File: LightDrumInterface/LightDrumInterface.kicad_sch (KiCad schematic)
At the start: 63 parts, among them J1 MIDI-IN, J2 DEBUG-CONN, J3 MIDI-OUT, J4 PWR-CONN, J5 0525593652, J6 0541323662, Q101 NX6008NBKWX, Q102 NX6008NBKWX, Q103 NX6008NBKWX, Q104 NX6008NBKWX, SW1 RESET-SW, U1 STP16CP05, U2 TPL0401B-10-Q1, U3 74AUP2G04, U4 PC817

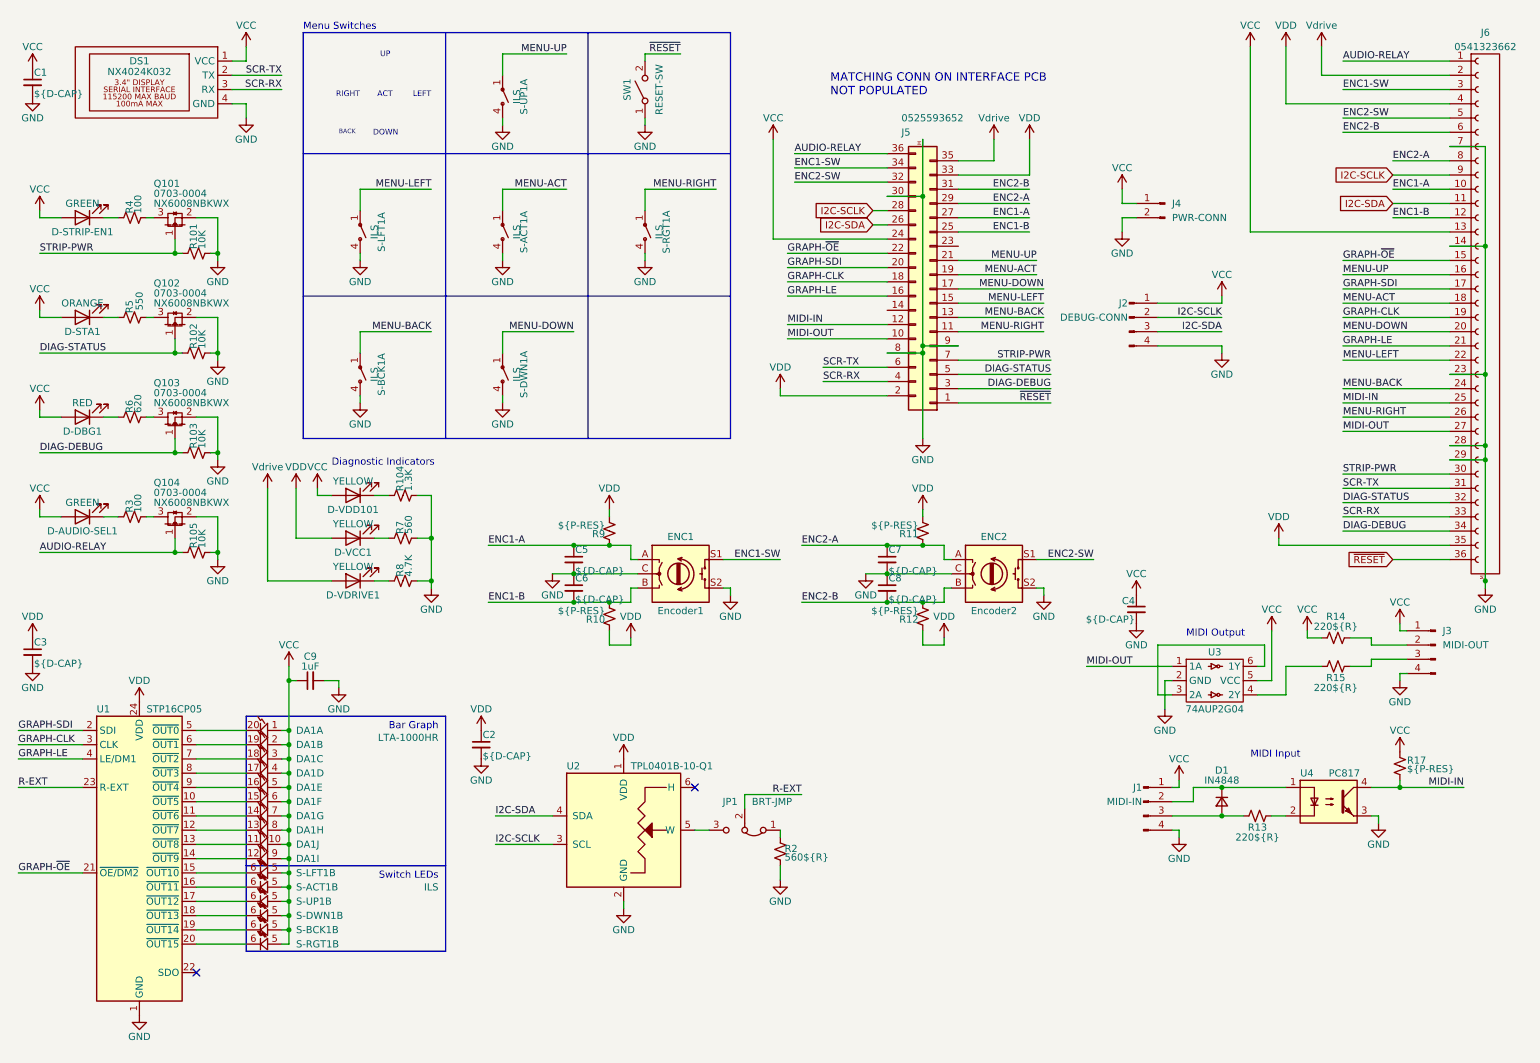
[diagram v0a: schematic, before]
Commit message: interface layout completed - REV6
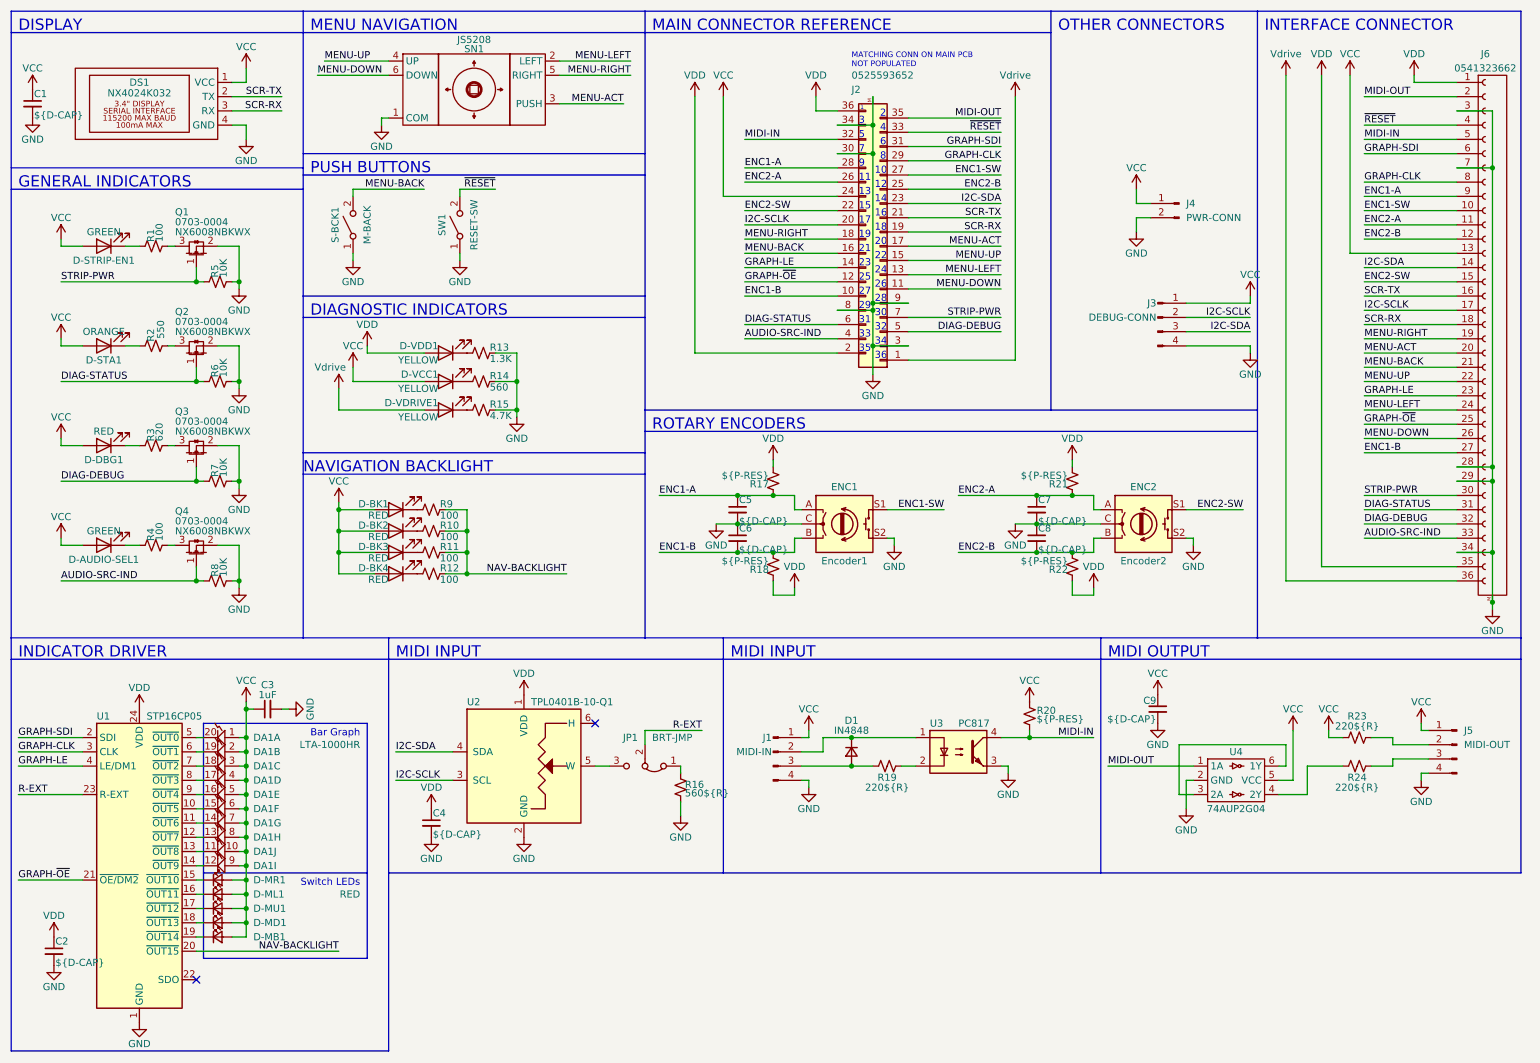
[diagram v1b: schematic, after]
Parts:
- removed S-ACT1, S-BCK1, S-DWN1, S-LFT1, S-RGT1, S-UP1: ILS, Daxxn_Switches:ILS-TB, symbol Daxxn_Buttons:ILS
- added D-BK1, D-BK2, D-BK3, D-BK4: RED, LED_SMD:LED_0805_2012Metric, symbol Device:LED
- added D-MB1, D-MD1, D-ML1, D-MR1, D-MU1: RED, LED_SMD:LED_0805_2012Metric, symbol Device:LED_Small
- added R10, R11, R12, R9: 100, Resistor_SMD:R_0805_2012Metric, symbol Device:R_Small_US
- added S-BCK1: M-BACK, Daxxn_Switches:TL3365AF180QG, symbol Switch:SW_SPST
- added SN1: JS5208, Daxxn_Switches:JS5208, symbol Daxxn_Buttons:JS5208
- DS1: footprint Daxxn_Displays:NX4024T032_10mm -> Daxxn_Displays:NX4024K032-RA-S04B
- ENC1, ENC2: footprint Daxxn_Switches:PEC12R -> Daxxn_Switches:PEC11R
- renumbered C3 to C2, C9 to C3, C2 to C4, C4 to C9, D-VDD101 to D-VDD1, J5 to J2, J2 to J3, J3 to J5, Q101 to Q1, Q102 to Q2, Q103 to Q3, Q104 to Q4, R4 to R1, R104 to R13, R7 to R14, R8 to R15, R2 to R16, R9 to R17, R10 to R18, R13 to R19, R5 to R2, R17 to R20, R11 to R21, R12 to R22, R14 to R23, R15 to R24, R6 to R3, R3 to R4, R101 to R5, R102 to R6, R103 to R7, R105 to R8, U4 to U3, U3 to U4
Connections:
- net DIAG-DEBUG: now also J2.5 (Pin_5), J6.32 (Pin_32); no longer J2.3 (Pin_3), J6.34 (Pin_34)
- net DIAG-STATUS: now also J2.6 (Pin_6), J6.31 (Pin_31); no longer J2.5 (Pin_5), J6.32 (Pin_32)
- net ENC1-A: now also J2.28 (Pin_28), J6.9 (Pin_9); no longer J2.27 (Pin_27), J6.10 (Pin_10)
- net ENC1-B: now also J2.10 (Pin_10), J6.27 (Pin_27); no longer J2.25 (Pin_25), J6.12 (Pin_12)
- net ENC1-SW: now also J2.27 (Pin_27), J6.10 (Pin_10); no longer J2.34 (Pin_34), J6.3 (Pin_3)
- net ENC2-A: now also J2.26 (Pin_26), J6.11 (Pin_11); no longer J2.29 (Pin_29), J6.8 (Pin_8)
- net ENC2-B: now also J2.25 (Pin_25), J6.12 (Pin_12); no longer J2.31 (Pin_31), J6.6 (Pin_6)
- net ENC2-SW: now also J2.22 (Pin_22), J6.15 (Pin_15); no longer J2.32 (Pin_32), J6.5 (Pin_5)
- net GND: now also J2.3 (Pin_3), J2.34 (Pin_34), J6.3 (Pin_3), J6.34 (Pin_34), S-BCK1.1 (A), SN1.1 (COM); no longer J6.14 (Pin_14), J6.23 (Pin_23)
- net GRAPH-CLK: now also J2.29 (Pin_29), J6.8 (Pin_8); no longer J2.18 (Pin_18), J6.19 (Pin_19)
- net GRAPH-LE: now also J2.14 (Pin_14), J6.23 (Pin_23); no longer J2.16 (Pin_16), J6.21 (Pin_21)
- net GRAPH-SDI: now also J2.31 (Pin_31), J6.6 (Pin_6); no longer J2.20 (Pin_20), J6.17 (Pin_17)
- net GRAPH-~{OE}: now also J2.12 (Pin_12), J6.25 (Pin_25); no longer J2.22 (Pin_22), J6.15 (Pin_15)
- net I2C-SCLK: now also J2.20 (Pin_20), J6.17 (Pin_17); no longer J2.28 (Pin_28), J6.9 (Pin_9)
- net I2C-SDA: now also J2.23 (Pin_23), J6.14 (Pin_14); no longer J2.26 (Pin_26), J6.11 (Pin_11)
- net MENU-ACT: now also J2.17 (Pin_17), J6.20 (Pin_20), SN1.3 (PUSH); no longer J2.19 (Pin_19), J6.18 (Pin_18)
- net MENU-BACK: now also J2.16 (Pin_16), J6.21 (Pin_21), S-BCK1.2 (B); no longer J2.13 (Pin_13), J6.24 (Pin_24)
- net MENU-DOWN: now also J2.11 (Pin_11), J6.26 (Pin_26), SN1.6 (DOWN); no longer J2.17 (Pin_17), J6.20 (Pin_20)
- net MENU-LEFT: now also J2.13 (Pin_13), J6.24 (Pin_24), SN1.2 (LEFT); no longer J2.15 (Pin_15), J6.22 (Pin_22)
- net MENU-RIGHT: now also J2.18 (Pin_18), J6.19 (Pin_19), SN1.5 (RIGHT); no longer J2.11 (Pin_11), J6.26 (Pin_26)
- net MENU-UP: now also J2.15 (Pin_15), J6.22 (Pin_22), SN1.4 (UP); no longer J2.21 (Pin_21), J6.16 (Pin_16)
- net MIDI-IN: now also J2.32 (Pin_32), J6.5 (Pin_5); no longer J2.12 (Pin_12), J6.25 (Pin_25)
- net MIDI-OUT: now also J2.35 (Pin_35), J6.2 (Pin_2); no longer J2.10 (Pin_10), J6.27 (Pin_27)
- net SCR-RX: now also J2.19 (Pin_19), J6.18 (Pin_18); no longer J2.4 (Pin_4), J6.33 (Pin_33)
- net SCR-TX: now also J2.21 (Pin_21), J6.16 (Pin_16); no longer J2.6 (Pin_6), J6.31 (Pin_31)
- net VCC: now also D-VCC1.2 (A), D-BK1.2 (A), D-BK2.2 (A), D-BK3.2 (A), D-BK4.2 (A), D-MB1.2 (A), D-MD1.2 (A), D-ML1.2 (A), D-MR1.2 (A), D-MU1.2 (A); no longer D-VDD1.2 (A)
- net VDD: now also D-VDD1.2 (A), J2.36 (Pin_36), J6.1 (Pin_1); no longer D-VCC1.2 (A), J2.33 (Pin_33), J6.4 (Pin_4)
- net Vdrive: now also J2.1 (Pin_1), J6.36 (Pin_36); no longer J2.35 (Pin_35), J6.2 (Pin_2)
- net ~{RESET}: now also J2.33 (Pin_33), J6.4 (Pin_4); no longer J2.1 (Pin_1), J6.36 (Pin_36)
- net at U1.19 (~{OUT14}): now also D-MB1.1 (K)
- net at U1.18 (~{OUT13}): now also D-MD1.1 (K)
- net NAV-BACKLIGHT: now reaches U1.20 (~{OUT15})
- net NAV-BACKLIGHT: now also R10.2, R11.2, R12.2, R9.2
- net at U1.15 (~{OUT10}): now also D-MR1.1 (K)
- net at U1.16 (~{OUT11}): now also D-ML1.1 (K)
- net at U1.17 (~{OUT12}): now also D-MU1.1 (K)
- net AUDIO-RELAY renamed AUDIO-SRC-IND
- net AUDIO-SRC-IND: now also J2.4 (Pin_4), J6.33 (Pin_33); no longer J2.36 (Pin_36), J6.1 (Pin_1)
- new net: D-BK3.1 (K), R11.1
- new net: D-BK2.1 (K), R10.1
- new net: D-BK1.1 (K), R9.1
- new net: D-BK4.1 (K), R12.1
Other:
- note added: "1"
- note added: "10"
- note added: "11"
- note added: "12"
- note added: "13"
- note added: "14"
- note added: "15"
- note added: "16"
- note added: "17"
- note added: "18"
- note added: "19"
- note added: "2"
- note added: "20"
- note added: "21"
- note added: "22"
- note added: "23"
- note added: "24"
- note added: "25"
- note added: "26"
- note added: "27"
- note added: "28"
- note added: "29"
- note added: "3"
- note added: "30"
- note added: "31"
- note added: "32"
- note added: "33"
- note added: "34"
- note added: "35"
- note added: "36"
- note added: "4"
- note added: "5"
- note added: "6"
- note added: "7"
- note added: "8"
- note added: "9"
- note added: "DIAGNOSTIC INDICATORS"
- note added: "DISPLAY"
- note added: "GENERAL INDICATORS"
- note added: "INDICATOR DRIVER"
- note added: "INTERFACE CONNECTOR"
- note added: "MAIN CONNECTOR REFERENCE"
- note added: "MATCHING CONN ON MAIN PCB NOT POPULATED"
- note added: "MENU NAVIGATION"
- note added: "MIDI INPUT"
- note added: "MIDI OUTPUT"
- note added: "NAVIGATION BACKLIGHT"
- note added: "OTHER CONNECTORS"
- note added: "PUSH BUTTONS"
- note added: "ROTARY ENCODERS"
- note removed: "ACT"
- note removed: "BACK"
- note removed: "DOWN"
- note removed: "Diagnostic Indicators"
- note removed: "LEFT"
- note removed: "MATCHING CONN ON INTERFACE PCB NOT POPULATED"
- note removed: "MIDI Input"
- note removed: "MIDI Output"
- note removed: "Menu Switches"
- note removed: "RIGHT"
- note removed: "UP"
- moved on the sheet: C1, C2, C3, C4, C5, C6, C7, C8, C9, D-AUDIO-SEL1, D-DBG1, D-STA1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
